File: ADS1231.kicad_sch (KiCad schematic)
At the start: 5 parts, among them J30 Conn_01x04, U12 ADS1231ID

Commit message: done ✅
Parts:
- J30: footprint (none) -> SM04B-GHS:JST_SM04B-GHS-TB_LF__SN_-
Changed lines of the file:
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@@
 			)
 		)
-		(property "Footprint" ""
+		(property "Footprint" "SM04B-GHS:JST_SM04B-GHS-TB_LF__SN_-"
 			(at 100.33 91.44 0)
 			(effects

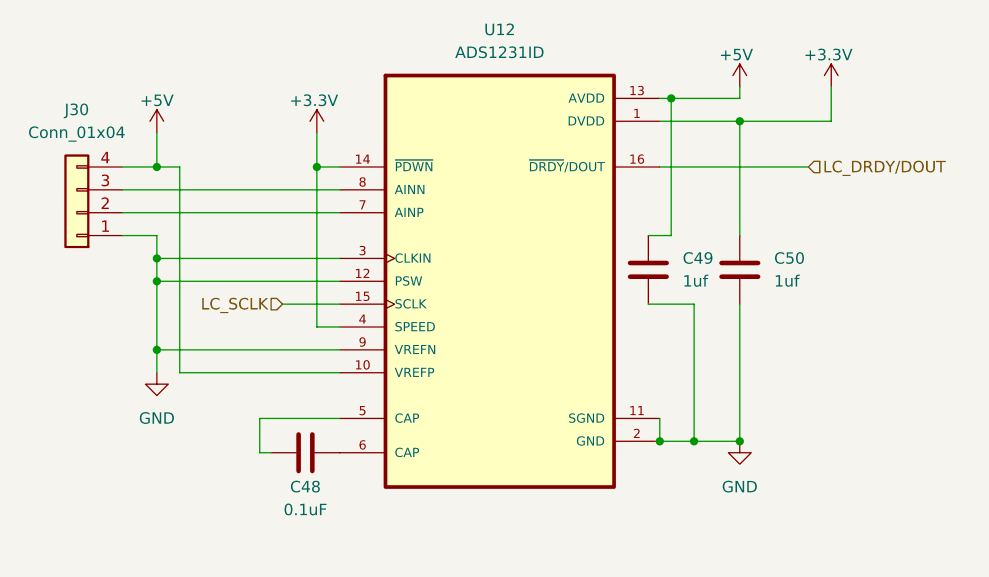
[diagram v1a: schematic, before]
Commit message: First Draft of BOM
Didn't select some compoentns like diodes that I don't fully understand. Also, some components have multiple variants so we must be careful.
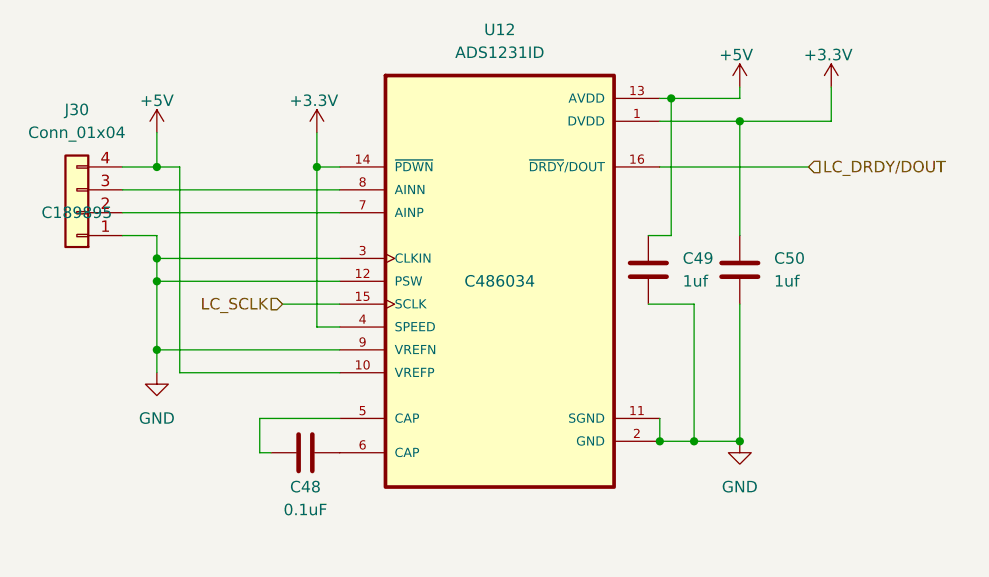
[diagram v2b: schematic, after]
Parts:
- J30: JLC# (none) -> C189895
- U12: JLC# (none) -> C486034
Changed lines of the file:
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@@
+			)
+		)
+		(property "JLC#" "C486034"
+			(at 147.32 99.06 0)
+			(effects
+				(font
+					(size 1.27 1.27)
+				)
 			)
 		)
@@
 				)
 				(hide yes)
+			)
+		)
+		(property "JLC#" ""
+			(at 125.73 118.11 0)
+			(effects
+				(font
+					(size 1.27 1.27)
+				)
 			)
 		)
@@
 			)
 		)
+		(property "JLC#" ""
+			(at 163.83 97.79 0)
+			(effects
+				(font
+					(size 1.27 1.27)
+				)
+			)
+		)
 		(pin "2"
 		)
@@
 			)
 		)
+		(property "JLC#" ""
+			(at 173.99 97.79 0)
+			(effects
+				(font
+					(size 1.27 1.27)
+				)
+			)
+		)
 		(pin "2"
 		)
@@
 			)
 		)
+		(property "JLC#" "C189895"
+			(at 100.33 91.44 0)
+			(effects
+				(font
+					(size 1.27 1.27)
+				)
+			)
+		)

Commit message: parts⚙️
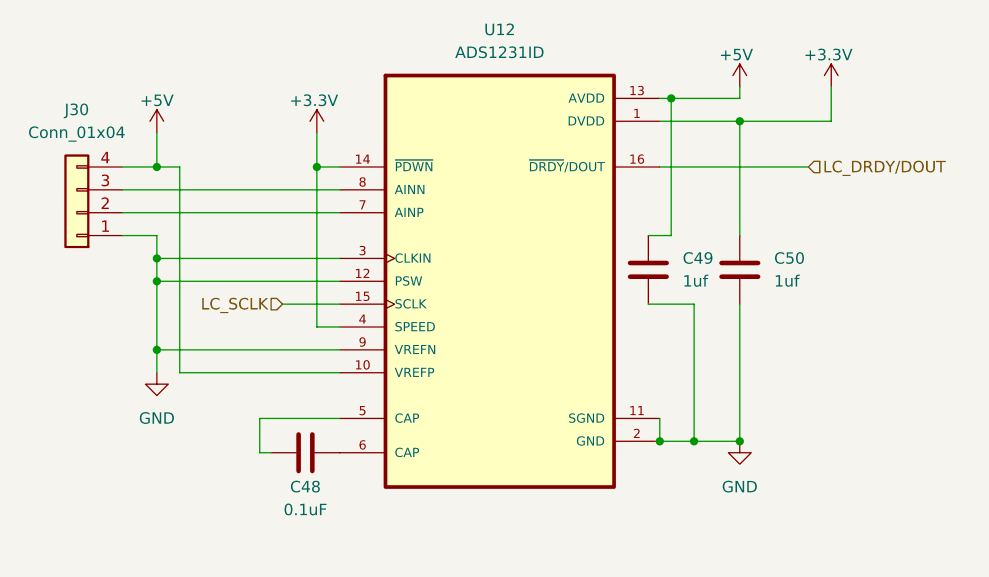
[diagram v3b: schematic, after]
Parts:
- U12: JLC# C486034 -> C486034
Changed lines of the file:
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@@
 			)
 		)
-		(property "JLC#" "C486034"
+		(property "JLC#" "C486034 "
 			(at 147.32 99.06 0)
 			(effects
@@
 					(size 1.27 1.27)
 				)
+				(hide yes)
 			)
 		)
@@
 					(size 1.27 1.27)
 				)
-			)
-		)
+				(hide yes)
+			)
+		)

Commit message: Initial pass at finding Mouser part numbers
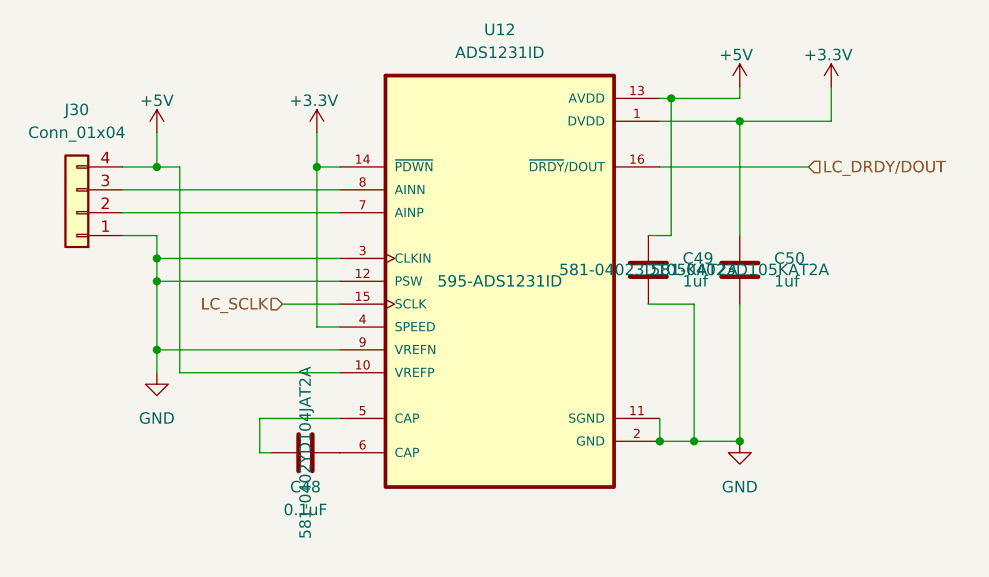
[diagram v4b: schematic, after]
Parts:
- C48: Mouser Part Number  (none) -> 581-0402YD104JAT2A
- C49, C50: Mouser Part Number  (none) -> 581-04023D105KAT2A
- U12: Mouser Part Number  (none) -> 595-ADS1231ID
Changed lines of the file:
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@@
+			)
+		)
+		(property "Mouser Part Number " "595-ADS1231ID "
+			(at 147.32 99.06 0)
+			(effects
+				(font
+					(size 1.27 1.27)
+				)
 			)
 		)
@@
 		)
 		(property "JLC#" ""
+			(at 125.73 118.11 0)
+			(effects
+				(font
+					(size 1.27 1.27)
+				)
+			)
+		)
+		(property "Mouser Part Number " "581-0402YD104JAT2A "
 			(at 125.73 118.11 0)
 			(effects
@@
 			)
 		)
+		(property "Mouser Part Number " "581-04023D105KAT2A "
+			(at 163.83 97.79 0)
+			(effects
+				(font
+					(size 1.27 1.27)
+				)
+			)
+		)
 		(pin "2"
 		)
@@
 			)
 		)
+		(property "Mouser Part Number " "581-04023D105KAT2A "
+			(at 173.99 97.79 0)
+			(effects
+				(font
+					(size 1.27 1.27)
+				)
+			)
+		)
 		(pin "2"
 		)
@@
 			)
 		)
+		(property "Mouser Part Number " ""
+			(at 100.33 91.44 0)
+			(effects
+				(font
+					(size 1.27 1.27)
+				)
+			)
+		)
